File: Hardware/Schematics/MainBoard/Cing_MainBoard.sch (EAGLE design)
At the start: 186 parts, among them IC1 L293D, IC2 LM2576S, IC3 FT232RL, IC4 BMP280, IC5 BME280, Q1 16mhz, Q2 BSS138, Q3 BSS138, Q4 BSS138, Q5 BSS138, Q6 NP2301AMR-G, Q7 NP2301AMR-G, T1 FS8205, T2 FS8205, U3 MPU-6050MPU6050, U4 CH330N

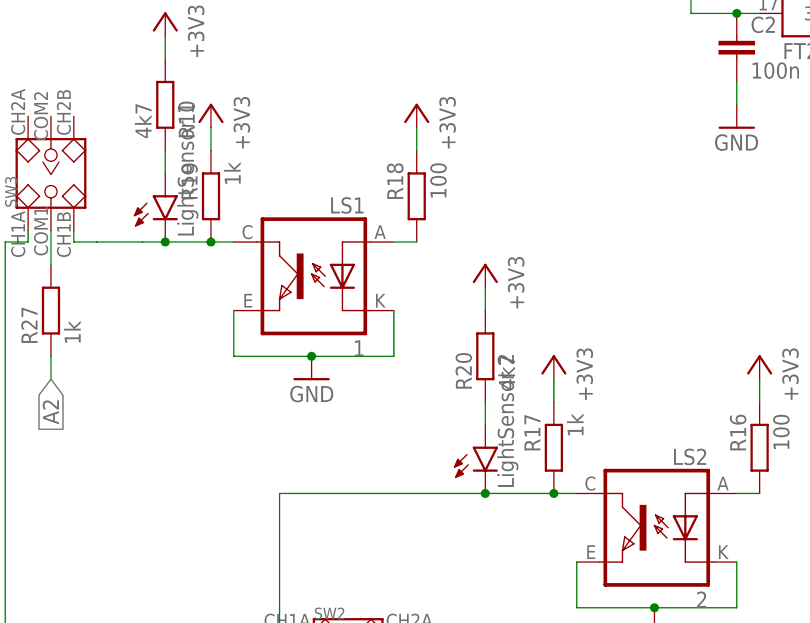
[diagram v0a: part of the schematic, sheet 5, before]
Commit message: modifications
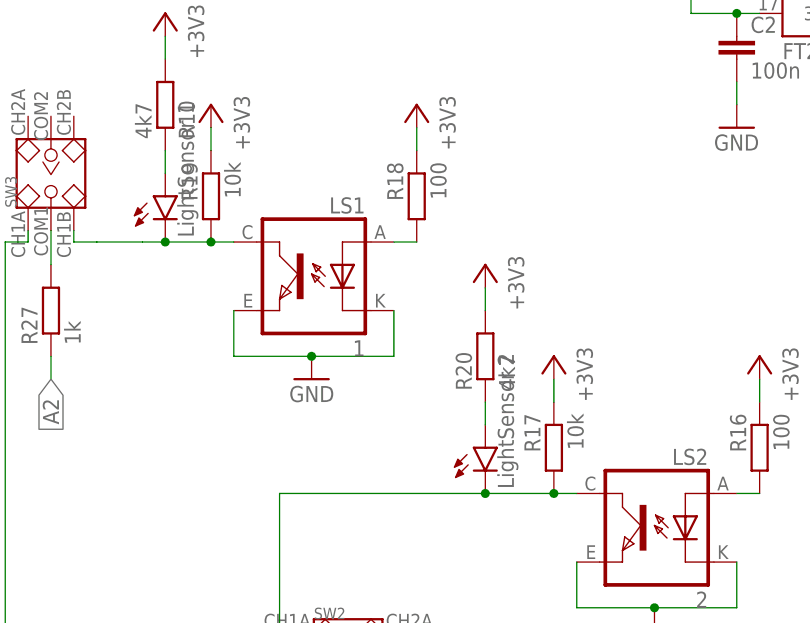
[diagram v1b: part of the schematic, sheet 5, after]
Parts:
- R17, R19: value 1k -> 10k
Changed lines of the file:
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@@
 <drawing>
 <settings>
-<setting alwaysvectorfont="yes"/>
+<setting alwaysvectorfont="no"/>
 <setting keepoldvectorfont="yes"/>
 <setting verticaltext="up"/>
@@
 <part name="GND16" library="supply1" library_urn="urn:adsk.eagle:library:371" deviceset="GND" device=""/>
 <part name="R16" library="rcl" library_urn="urn:adsk.eagle:library:334" deviceset="R-EU_" device="R1206" package3d_urn="urn:adsk.eagle:package:23540/2" override_package3d_urn="urn:adsk.eagle:package:11835280/2" override_package_urn="urn:adsk.eagle:footprint:23047/1" value="100"/>
-<part name="R17" library="rcl" library_urn="urn:adsk.eagle:library:334" deviceset="R-EU_" device="R1206" package3d_urn="urn:adsk.eagle:package:23540/2" override_package3d_urn="urn:adsk.eagle:package:11835281/2" override_package_urn="urn:adsk.eagle:footprint:23047/1" value="1k"/>
+<part name="R17" library="rcl" library_urn="urn:adsk.eagle:library:334" deviceset="R-EU_" device="R1206" package3d_urn="urn:adsk.eagle:package:23540/2" override_package3d_urn="urn:adsk.eagle:package:11835281/2" override_package_urn="urn:adsk.eagle:footprint:23047/1" value="10k"/>
 <part name="GND18" library="supply1" library_urn="urn:adsk.eagle:library:371" deviceset="GND" device=""/>
 <part name="R18" library="rcl" library_urn="urn:adsk.eagle:library:334" deviceset="R-EU_" device="R1206" package3d_urn="urn:adsk.eagle:package:23540/2" value="100"/>
-<part name="R19" library="rcl" library_urn="urn:adsk.eagle:library:334" deviceset="R-EU_" device="R1206" package3d_urn="urn:adsk.eagle:package:23540/2" override_package3d_urn="urn:adsk.eagle:package:11835296/2" override_package_urn="urn:adsk.eagle:footprint:23047/1" value="1k"/>
+<part name="R19" library="rcl" library_urn="urn:adsk.eagle:library:334" deviceset="R-EU_" device="R1206" package3d_urn="urn:adsk.eagle:package:23540/2" override_package3d_urn="urn:adsk.eagle:package:11835296/2" override_package_urn="urn:adsk.eagle:footprint:23047/1" value="10k"/>
 <part name="GND13" library="supply1" library_urn="urn:adsk.eagle:library:371" deviceset="GND" device=""/>
 <part name="R3" library="rcl" library_urn="urn:adsk.eagle:library:334" deviceset="R-EU_" device="R1206" package3d_urn="urn:adsk.eagle:package:23540/2" override_package3d_urn="urn:adsk.eagle:package:11835130/2" override_package_urn="urn:adsk.eagle:footprint:23047/1" value="40"/>
